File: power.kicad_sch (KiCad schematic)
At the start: 6 parts, among them U50 LDL1117S33R, U52 MIC5219-2.85YM5-TR

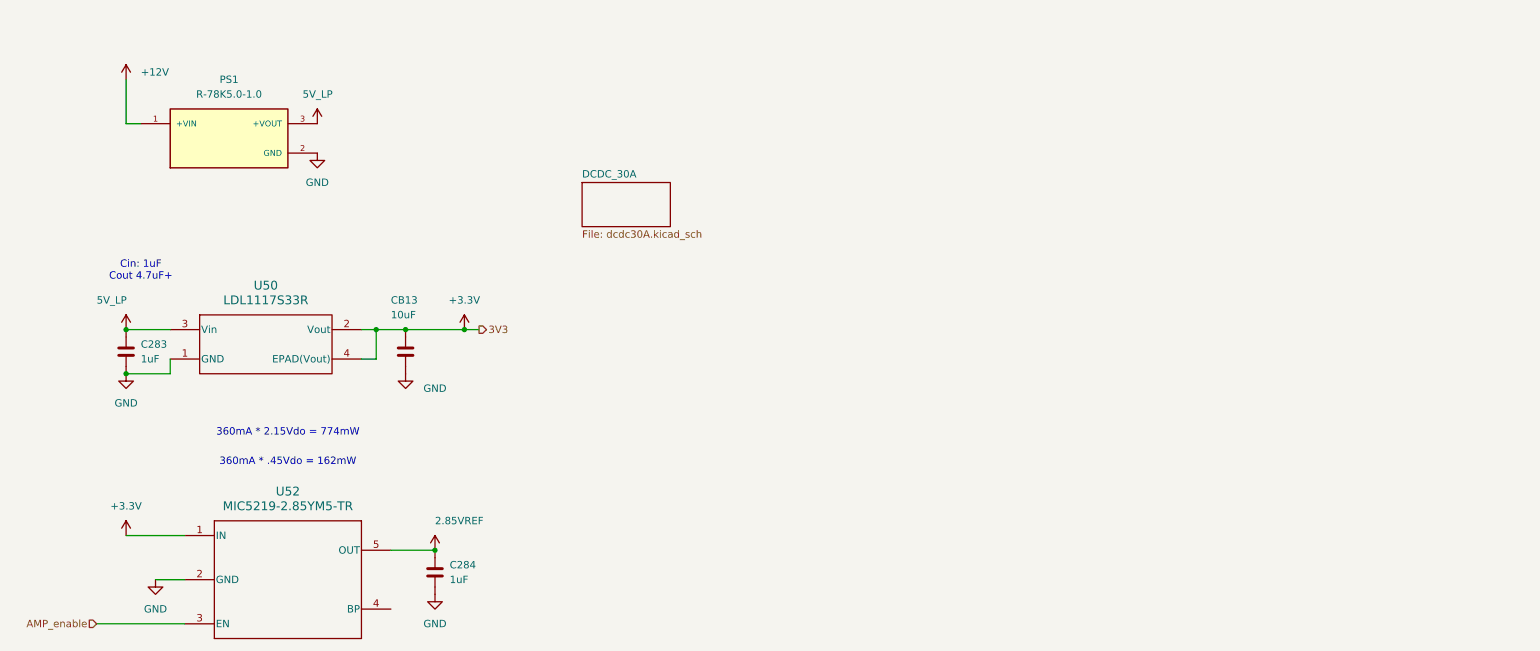
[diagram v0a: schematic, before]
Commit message: moving along
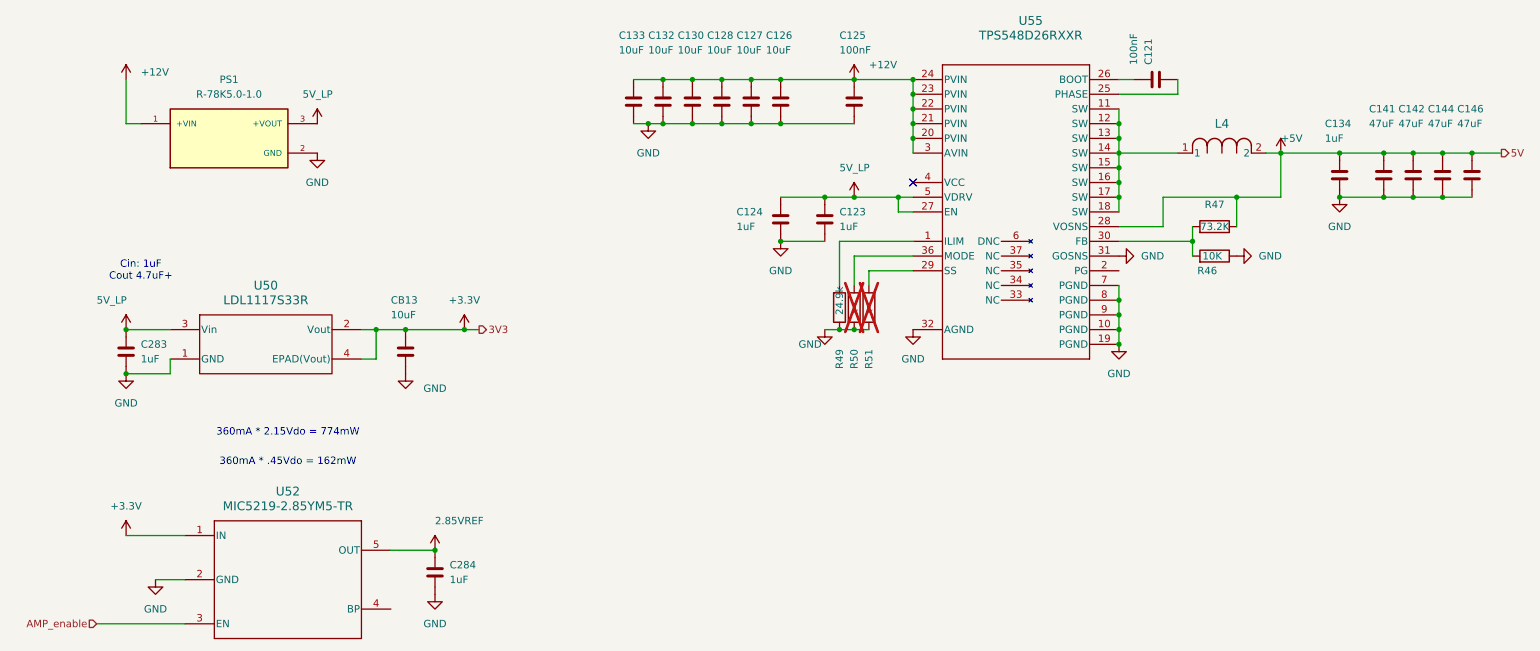
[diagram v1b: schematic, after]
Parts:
- added C121, C125: 100nF, Capacitor_SMD:C_0603_1608Metric, symbol Capacitors:0603_nf100
- added C123, C124, C134: 1uF, Capacitor_SMD:C_0603_1608Metric, symbol Capacitors:0603_uF001_50V
- added C126, C127, C128, C130, C132, C133: 10uF, Capacitor_SMD:C_1206_3216Metric, symbol Capacitors:1206_uF010
- added C141, C142, C144, C146: 47uF, Capacitor_SMD:C_1206_3216Metric, symbol Capacitors:1206_uF010
- added L4: IHLP6767GZERR47M11, Inductors:IND_IHLP-6767GZ_VIS, symbol Inductors:IHLP6767GZERR47M11
- added R46: 10K, Resistor_SMD:R_0603_1608Metric, symbol Resistors:0603_R_10K
- added R47: 73.2K, Resistor_SMD:R_0603_1608Metric, symbol Resistors:0603_R_73K2
- added R49: 24.9k, Resistor_SMD:R_0603_1608Metric, symbol Resistors:0603_R_52K3
- added R50, R51: x, Resistor_SMD:R_0603_1608Metric, symbol Resistors:0603_R_52K3
- added U55: TPS548D26RXXR, DCDC:WQFN_C26RXXR_TEX, symbol DCDC:TPS548C26RXXR
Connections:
- net +12V: now also C125.1, C126.1, C127.1, C128.1, C130.1, C132.1, C133.1, U55.20 (PVIN), U55.21 (PVIN), U55.22 (PVIN), U55.23 (PVIN), U55.24 (PVIN), U55.3 (AVIN)
- net 5V_LP: now also C123.1, C124.1, U55.27 (EN), U55.5 (VDRV)
- net GND: now also C123.2, C124.2, C125.2, C126.2, C127.2, C128.2, C130.2, C132.2, C133.2, C134.2, C141.2, C142.2, C144.2, C146.2, R46.2, R49.2, R50.2, R51.2, U55.10 (PGND), U55.19 (PGND), U55.31 (GOSNS), U55.32 (AGND), U55.7 (PGND), U55.8 (PGND), U55.9 (PGND)
- new net: R50.1, U55.36 (MODE)
- new net: R49.1, U55.1 (ILIM)
- new net: R46.1, R47.1, U55.30 (FB)
- new net: L4.1, U55.11 (SW), U55.12 (SW), U55.13 (SW), U55.14 (SW), U55.15 (SW), U55.16 (SW), U55.17 (SW), U55.18 (SW)
- new net: C121.2, U55.25 (PHASE)
- new net: C121.1, U55.26 (BOOT)
- new net: R51.1, U55.29 (SS)
- new net +5V: C134.1, C141.1, C142.1, C144.1, C146.1, L4.2, R47.2, U55.28 (VOSNS)
- no-connect marks 0 -> 1
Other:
- removed sheet DCDC_30A
